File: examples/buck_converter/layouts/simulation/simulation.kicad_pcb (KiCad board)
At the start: 2 copper layers, 14 parts

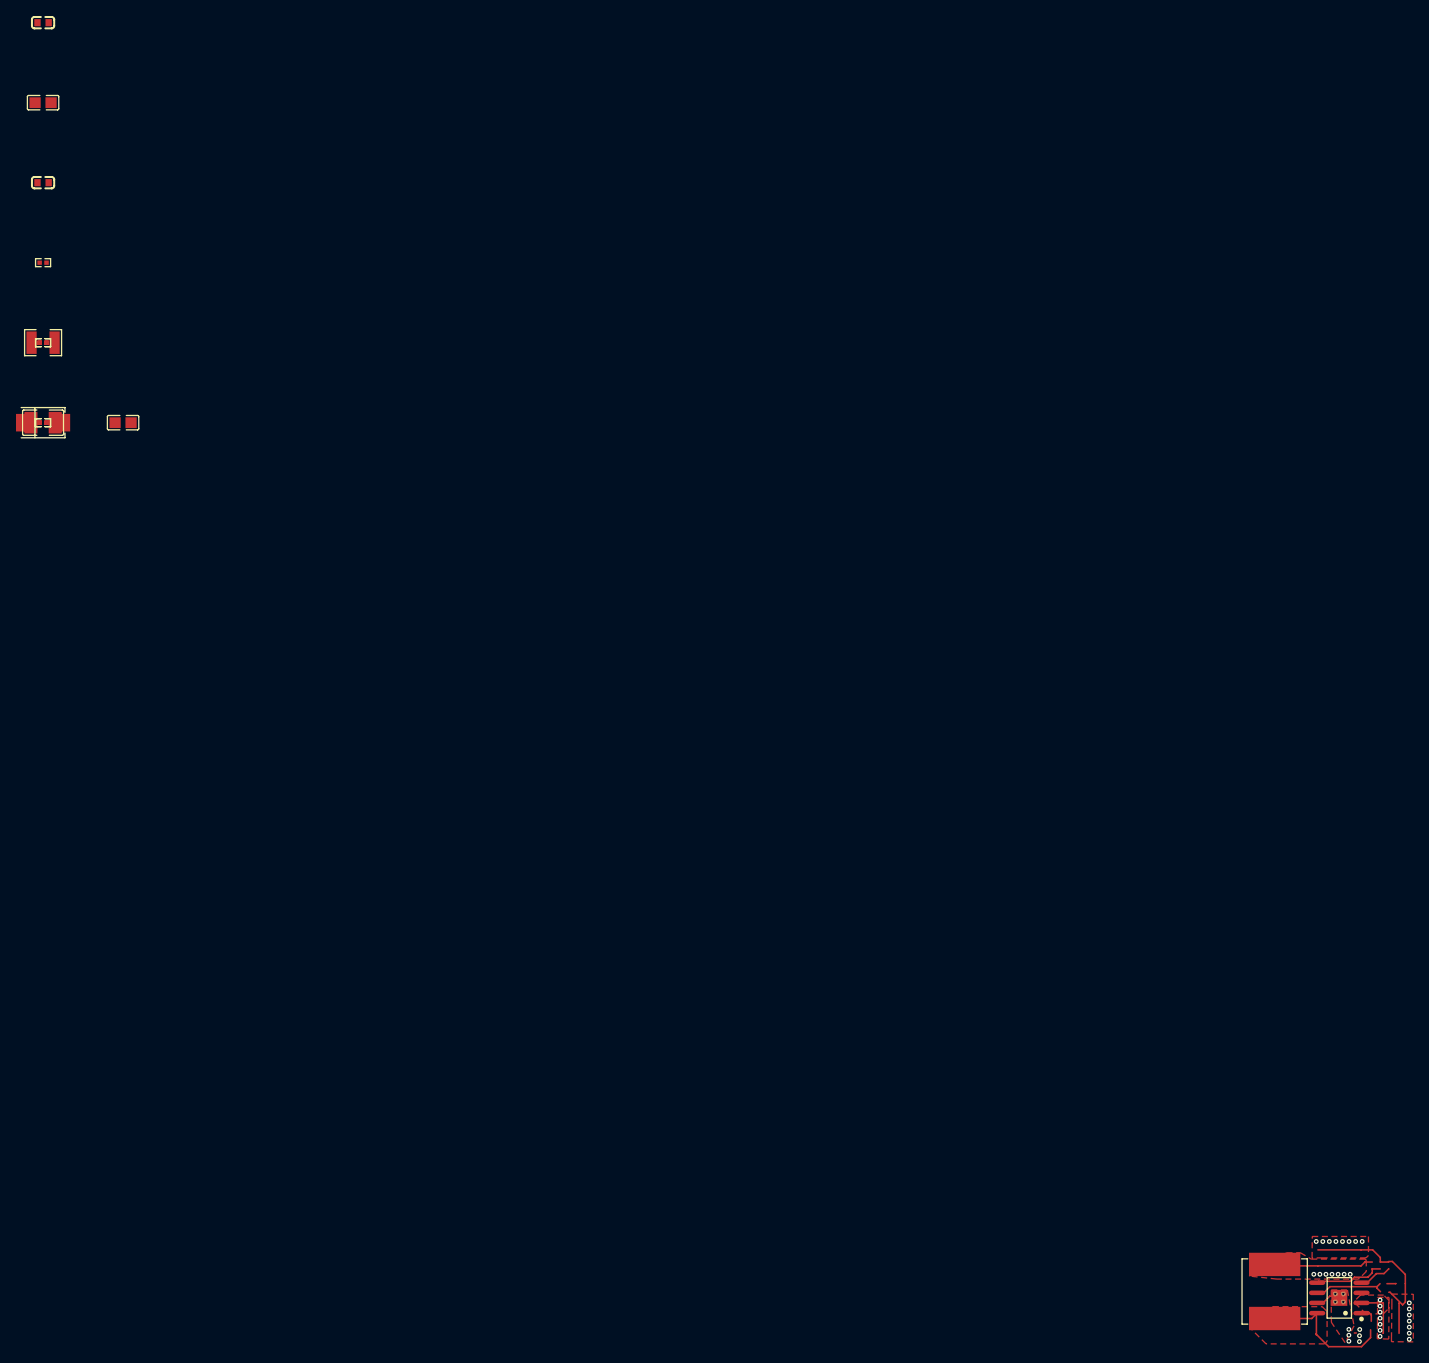
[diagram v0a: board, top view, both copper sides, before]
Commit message: final checkin
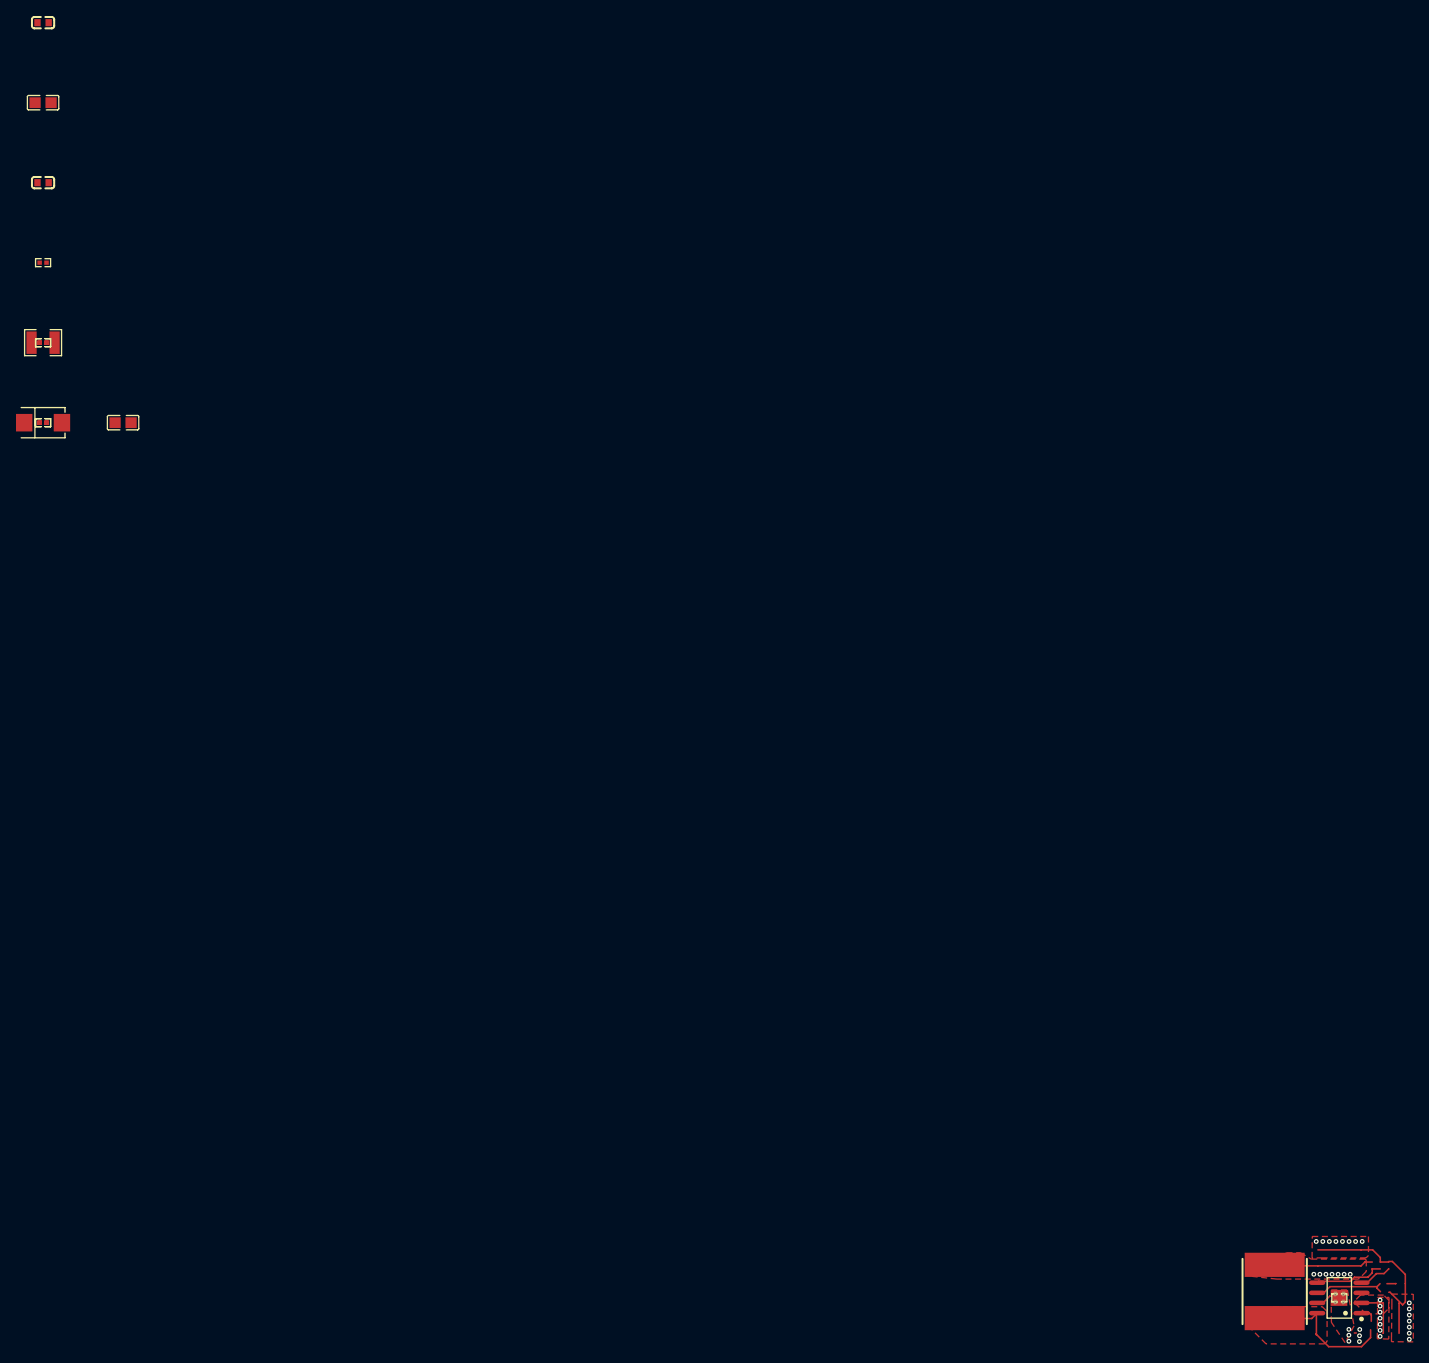
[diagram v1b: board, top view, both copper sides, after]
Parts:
- removed C5: 0F, Chinocera_HGC1210R5107M160NSVK:C1210
- added R7: 91000Ω, YAGEO_RC0402FR_0791KL:R0402, F.Cu at (0.00, 0.00)
- C2: footprint YAGEO_CC0603JRNPO9BN8R2:C0603 -> Samsung_Electro_Mechanics_CL10C470JB8NNNC:C0603
- C3: footprint FH_0805B333K500NT:C0805 -> FH_0805B472K500NT:C0805
- L1: footprint Sunlord_SWPA8040S2R2MT:IND-SMD_L8.0-W8.0_SWPA8040S -> YJYCOIN_YNR8040_6R8M:IND-SMD_L8.0-W8.0
- R1: value 7680Ω -> 10200Ω; footprint UNI_ROYAL_0402WGF7681TCE:R0402 -> UNI_ROYAL_0402WGF1022TCE:R0402
- R2: value 23700Ω -> 16900Ω; footprint YAGEO_RC0402FR_0723K7L:R0402 -> UNI_ROYAL_0402WGF1692TCE:R0402
- R3: value 100000Ω -> 450000Ω; footprint UNI_ROYAL_0402WGF1003TCE:R0402 -> FOJAN_FRC0402F4503TS:R0402
- R5: value 95300Ω -> 243000Ω; footprint Vishay_Intertech_CRCW040295K3FKED:R0402 -> UNI_ROYAL_0402WGF2433TCE:R0402
- R6: value 40200Ω -> 53600Ω; footprint UNI_ROYAL_0402WGF4022TCE:R0402 -> UNI_ROYAL_0402WGF5362TCE:R0402
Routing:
- net power_out-hv: track 26.8 -> 0.00 mm, vias 21 -> 0
- net 12: track 0.00 -> 26.8 mm, vias 0 -> 21
- net EN: track 2.06 -> 0.00 mm
- net 20: track 0.00 -> 2.06 mm
